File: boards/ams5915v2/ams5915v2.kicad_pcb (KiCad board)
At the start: 2 copper layers, 20.5 x 53 mm, 26 parts, among them J1 Conn_01x04, M3 MountingHole_3.2mm_M3, U1 MAX4995A, U2 TLV73333PDBVR, U3 AMS5915, U4 AMS5915

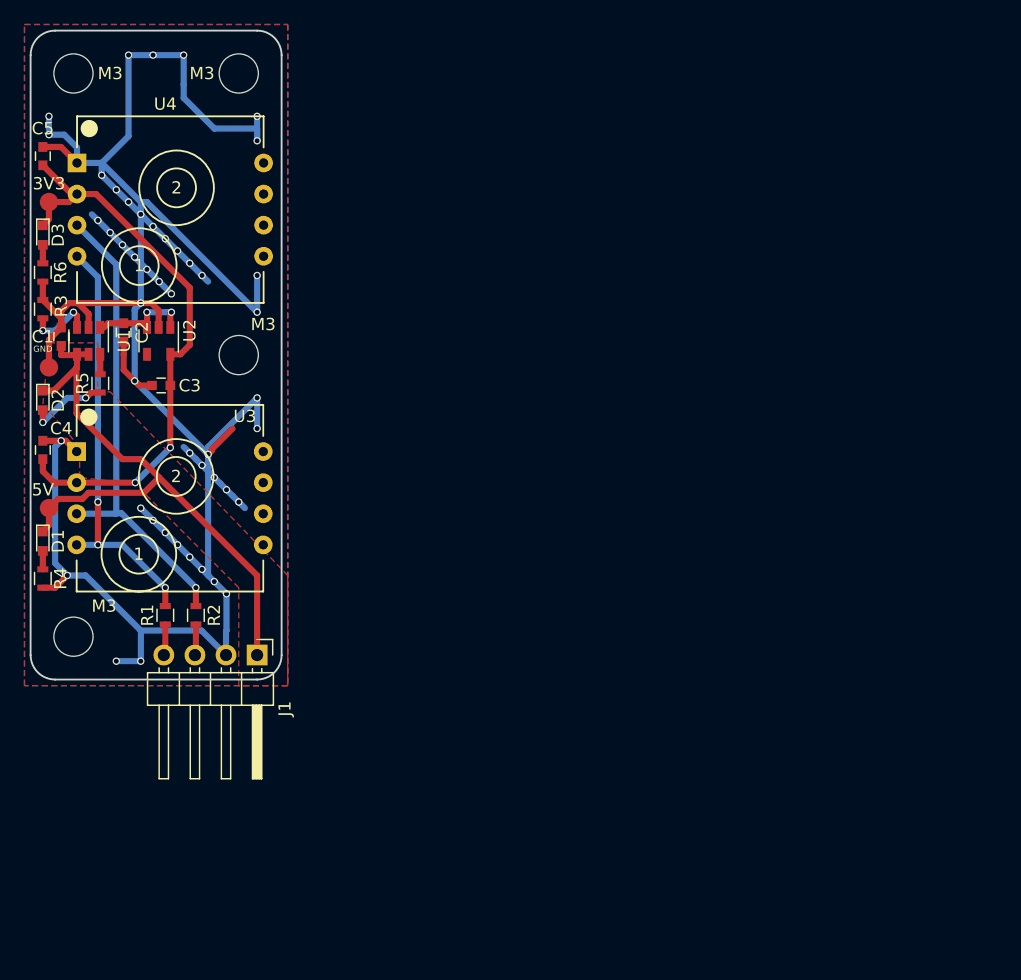
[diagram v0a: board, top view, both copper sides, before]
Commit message: ams5915x2: temp save
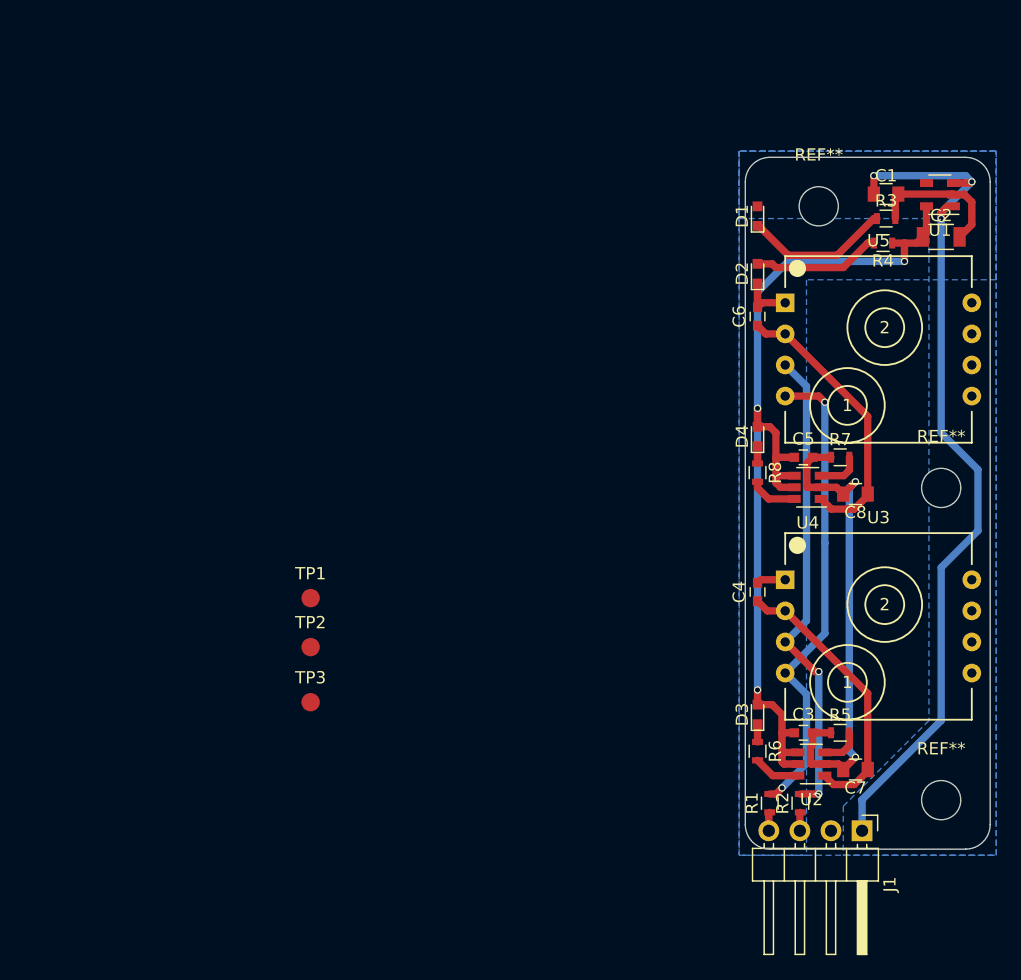
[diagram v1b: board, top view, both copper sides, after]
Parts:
- removed 3V3: 3v3, Measurement_Points:Measurement_Point_Round-SMD-Pad_Small
- removed 5V: 5v, Measurement_Points:Measurement_Point_Round-SMD-Pad_Small
- removed GND: GND, Measurement_Points:Measurement_Point_Round-SMD-Pad_Small
- removed M3 (x4): MountingHole_3.2mm_M3, Mounting_Holes:MountingHole_3.2mm_M3
- added C6: 100n, Capacitors_SMD:C_0603, F.Cu at (177.5, 82.0)
- added C7: 1u, Capacitors_SMD:C_0805, F.Cu at (185.5, 119.0)
- added C8: 1u, Capacitors_SMD:C_0805, F.Cu at (185.5, 96.5)
- added D4: LED_P2, LEDs:LED_0603, F.Cu at (177.5, 91.8)
- added R7: 400k, Resistors_SMD:R_0603, F.Cu at (184.2, 93.5)
- added R8: 2k7, Resistors_SMD:R_0603, F.Cu at (177.5, 94.8)
- added REF**: MountingHole_3.2mm_M3, Mounting_Holes:MountingHole_3.2mm_M3, F.Cu at (192.5, 96.0)
- added REF**: MountingHole_3.2mm_M3, Mounting_Holes:MountingHole_3.2mm_M3, F.Cu at (192.5, 121.5)
- added REF**: MountingHole_3.2mm_M3, Mounting_Holes:MountingHole_3.2mm_M3, F.Cu at (182.5, 73.0)
- added TP1: 5v, Measurement_Points:Measurement_Point_Round-SMD-Pad_Small, F.Cu at (141.0, 105.0)
- added TP2: GND, Measurement_Points:Measurement_Point_Round-SMD-Pad_Small, F.Cu at (141.0, 109.0)
- added TP3: 3v3, Measurement_Points:Measurement_Point_Round-SMD-Pad_Small, F.Cu at (141.0, 113.5)
- added U5: AMS5915, kicad-footprints-rchojetzki:AMS_5915-XXXX-D_differential_pressure_sensor, F.Cu at (179.8, 77.1)
- C1: footprint Capacitors_SMD:C_0603 -> Capacitors_SMD:C_0805
- C2: value 100n -> 10u; footprint Capacitors_SMD:C_0603 -> Capacitors_SMD:C_1206
- C3: value 1u -> 100n
- D1: value LED -> LED_5v
- D2: value LED -> LED_3v3
- D3: value LED -> LED_P1
- R3: value 300k -> 4k7
- R4, R6: value R -> 2k7
- R5: value R -> 400k
- U1: value MAX4995A -> TLV73333PDBVR; footprint TO_SOT_Packages_SMD:SOT-23-6 -> TO_SOT_Packages_SMD:SOT-23-5
- U2: value TLV73333PDBVR -> MAX4995A; footprint TO_SOT_Packages_SMD:SOT-23-5 -> TO_SOT_Packages_SMD:SOT-23-6
- U4: value AMS5915 -> MAX4995A; footprint kicad-footprints-rchojetzki:AMS_5915-XXXX-D_differential_pressure_sensor -> TO_SOT_Packages_SMD:SOT-23-6
- moved R4 73.9 mm to (187.8, 76.0), turned to 180 degrees
- moved U1 70.5 mm to (192.4, 72.0), turned to 180 degrees
- moved D3 70.3 mm to (177.5, 114.5), turned to 90 degrees
- moved R6 70.3 mm to (177.5, 117.5)
- moved R3 69.3 mm to (188.0, 74.0), turned to 0 degrees
- moved C1 68.4 mm to (188.0, 72.0), turned to 0 degrees
- moved C2 67.2 mm to (192.5, 75.5), turned to 0 degrees
- moved U4 66.9 mm to (181.6, 96.0), turned to 180 degrees
- moved R5 66.8 mm to (184.2, 116.0), turned to 0 degrees
- moved C5 66.8 mm to (181.2, 93.5), turned to 0 degrees
- moved D1 64.1 mm to (177.5, 73.8), turned to 90 degrees
- moved U2 63.5 mm to (181.9, 118.5), turned to 180 degrees
- moved C3 59.6 mm to (181.2, 116.0), turned to 0 degrees
- moved C4 59.5 mm to (177.5, 104.5)
- moved D2 59.3 mm to (177.5, 78.5), turned to 90 degrees
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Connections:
- C2 pad 1: /5vSWITCHED -> /3v3
- C4 pad 1: /3v3 -> Net-(C4-Pad1)
- D1 pad 1: /5v -> Net-(D1-Pad1)
- D1 pad 2: Net-(D1-Pad2) -> /5v
- D2 pad 1: /5v -> /GND
- D3 pad 1: /3v3 -> Net-(D3-Pad1)
- D3 pad 2: Net-(D3-Pad2) -> /3v3
- R3 pad 1: Net-(R3-Pad1) -> Net-(D1-Pad1)
- R4 pad 1: Net-(D1-Pad2) -> /3v3
- R4 pad 2: /GND -> Net-(D2-Pad2)
- R5 pad 1: Net-(D2-Pad2) -> /GND
- R6 pad 1: Net-(D3-Pad2) -> Net-(D3-Pad1)
- R6 pad 2: /GND -> Net-(R6-Pad2)
- U1 pad 1: /5vSWITCHED -> /5v
- U1 pad 3: Net-(R3-Pad1) -> /5v
- U1 pad 4: /5v -> Net-(U1-Pad4)
- U1 pad 5: /5v -> /3v3
- U2 pad 1: /5vSWITCHED -> Net-(C4-Pad1)
- U2 pad 3: /5vSWITCHED -> Net-(R5-Pad2)
- U2 pad 4: Net-(U2-Pad4) -> /3v3
- U3 pad 2: /3v3 -> Net-(C4-Pad1)
- U4 pad 1: /GND -> Net-(C6-Pad1)
- U4 pad 2: /3v3 -> /GND
- U4 pad 3: Net-(R2-Pad2) -> Net-(R7-Pad2)
- U4 pad 4: Net-(R1-Pad2) -> /3v3
- U4 pad 5: Net-(U4-Pad5) -> /3v3
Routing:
- net /GND: track 213.2 -> 58.4 mm, vias 47 -> 2
- net /3v3: track 48.1 -> 75.5 mm, vias 2 -> 3
- net Net-(C6-Pad1): track 0.00 -> 23.1 mm
- net Net-(C4-Pad1): track 0.00 -> 22.7 mm
- net /5v: track 50.3 -> 72.2 mm, vias 0 -> 3
- net Net-(D1-Pad1): track 0.00 -> 12.0 mm
- net /5vSWITCHED: track 8.62 -> 0.00 mm, vias 2 -> 0
- net Net-(R3-Pad1): track 5.48 -> 0.00 mm, vias 2 -> 0
- net Net-(R1-Pad2): track 34.5 -> 39.0 mm, vias 3 -> 2
- net Net-(R8-Pad2): track 0.00 -> 3.87 mm
- net Net-(R6-Pad2): track 0.00 -> 3.82 mm
- net Net-(D2-Pad2): track 6.70 -> 10.5 mm, vias 2 -> 0
- net Net-(R7-Pad2): track 0.00 -> 3.54 mm
- net Net-(R5-Pad2): track 1.62 -> 3.28 mm
- net Net-(D3-Pad2): track 1.50 -> 0.00 mm
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- added copper zone on B.Cu, net /3v3
- added copper zone on B.Cu, net /5v
- removed copper zone on F.Cu, net /5v
- removed copper zone on F.Cu, net /GND
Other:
- board size 20.5 x 53 mm -> 20 x 56.5 mm
- net class Default: trace_width 0.5 -> 0.6
- rule pad_to_mask_clearance: 0.2 -> 0
